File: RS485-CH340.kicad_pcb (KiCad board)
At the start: 2 copper layers, 22.5 x 14.5 mm, 13 parts, among them J1 USB_A, J2 Conn_01x04_Pin, U1 CH340N, U2 THVD1406DR

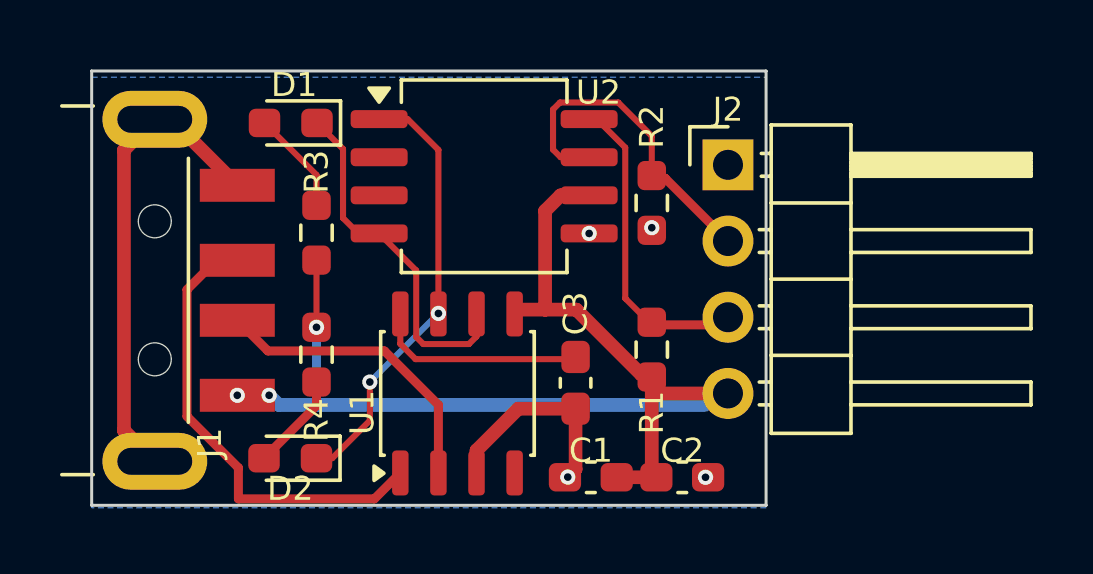
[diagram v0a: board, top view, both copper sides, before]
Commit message: Generate gerbers & fix C1/C2 overlapping courtyards
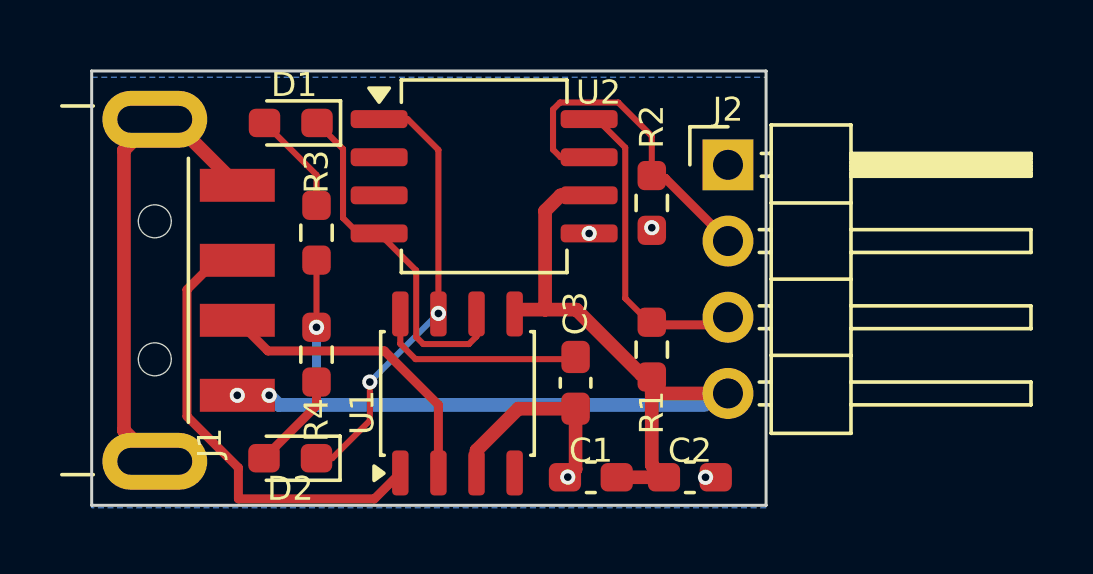
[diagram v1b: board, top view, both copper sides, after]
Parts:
- moved C2 0.25 mm to (149.4, 99.9)
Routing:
- net +5V: track 38.3 -> 39.2 mm
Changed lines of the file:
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@@
 			(outputformat 1)
 			(mirror no)
-			(drillshape 1)
+			(drillshape 0)
 			(scaleselection 1)
 			(outputdirectory "")
@@
 	(footprint "Capacitor_SMD:C_0603_1608Metric_Pad1.08x0.95mm_HandSolder"
 		(layer "F.Cu")
-		(at 149.098 99.949)
+		(at 149.352 99.949)
 		(descr "Capacitor SMD 0603 (1608 Metric), square (rectangular) end terminal, IPC-7351 nominal with elongated pad for handsoldering. (Body size source: IPC-SM-782 page 76, https://www.pcb-3d.com/wordpress/wp-content/uploads/ipc-sm-782a_amendment_1_and_2.pdf)")
 		(tags "capacitor handsolder")
@@
 	)
 	(segment
+		(start 148.4895 99.949)
+		(end 146.825 99.949)
+		(width 0.4572)
+		(layer "F.Cu")
+		(net "+5V")
+	)
+	(segment
 		(start 148.082 96.519)
 		(end 148.082 97.155)
@@
 	)
 	(segment
-		(start 148.2355 99.949)
-		(end 146.825 99.949)
-		(width 0.4572)
-		(layer "F.Cu")
-		(net "+5V")
-	)
-	(segment
 		(start 148.092 97.165)
 		(end 148.102 97.155)
@@
 	)
 	(segment
-		(start 148.082 99.7955)
-		(end 148.2355 99.949)
-		(width 0.4572)
-		(layer "F.Cu")
-		(net "+5V")
-	)
-	(segment
-		(start 148.082 97.155)
-		(end 148.082 99.7955)
+		(start 148.082 99.5415)
+		(end 148.4895 99.949)
 		(width 0.4572)
 		(layer "F.Cu")
@@
 		(width 0.4572)
 		(layer "F.Cu")
+		(net "+5V")
+	)
+	(segment
+		(start 148.082 96.6065)
+		(end 148.082 99.5415)
+		(width 0.4572)
+		(layer "F.Cu")
